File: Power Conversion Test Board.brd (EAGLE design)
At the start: 136.7 x 125.3 mm, 51 parts, among them U1 LM2678, U2 LM2678

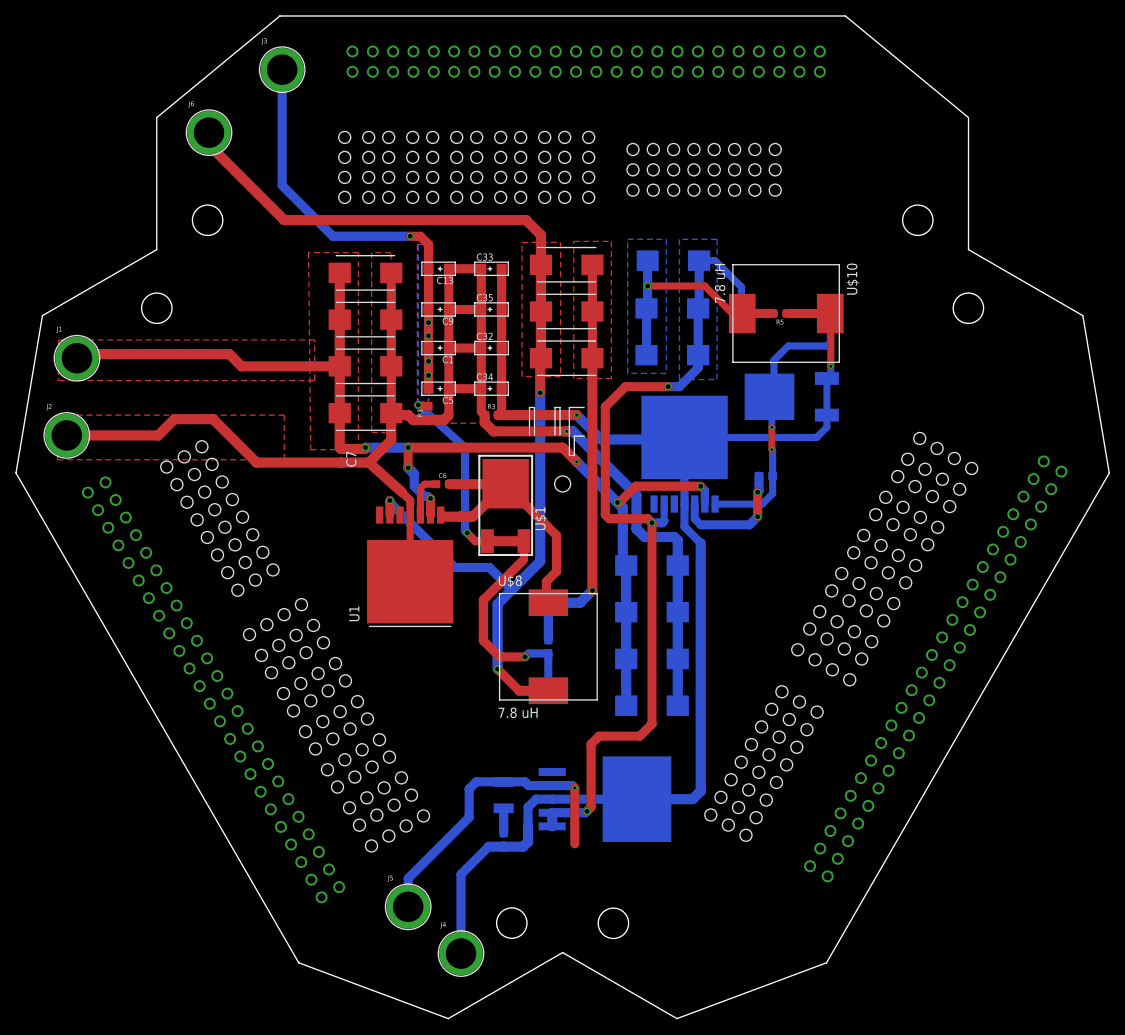
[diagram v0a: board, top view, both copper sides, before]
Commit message: Made some minor changes to the board, just uploading for saving purposes
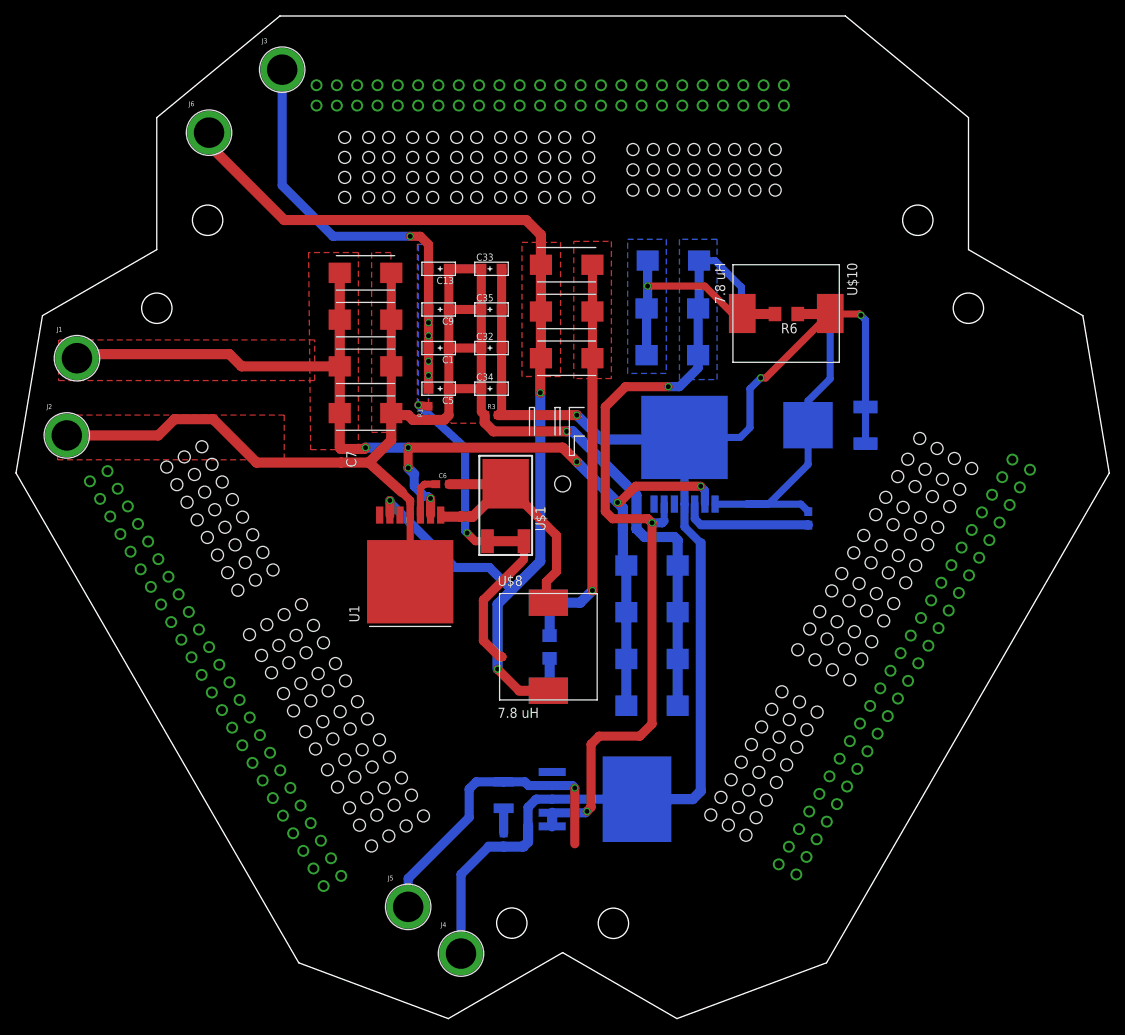
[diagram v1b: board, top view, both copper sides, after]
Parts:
- removed R2, R5: 0, SparkFun-Resistors:0603
- removed U$12, U$13, U$14: PDB_PCB_CONNEC, PDB_PCB_connectors:PDB_PCB
- added R6, R7: 0, audio amplifier example:R1206
- added U$2: PDB_PCB_CONNEC, PDB_PCB_connectors:PDB_PCB_2
- moved C20 7.49 mm to (99.0, 62.5), turned to 90 degrees
- moved U$3 5.99 mm to (102.1, 74.2)
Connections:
- net +12V: now also U$2.+12V1, U$2.+12V10, U$2.+12V11, U$2.+12V12, U$2.+12V13, U$2.+12V14, U$2.+12V15, U$2.+12V16, U$2.+12V17, U$2.+12V18, U$2.+12V19, U$2.+12V2, U$2.+12V20, U$2.+12V21, U$2.+12V22, U$2.+12V23, U$2.+12V24, U$2.+12V25, U$2.+12V26, U$2.+12V27, U$2.+12V28, U$2.+12V29, U$2.+12V3, U$2.+12V30, U$2.+12V31, U$2.+12V32, U$2.+12V33, U$2.+12V34, U$2.+12V35, U$2.+12V36, U$2.+12V37, U$2.+12V38, U$2.+12V39, U$2.+12V4, U$2.+12V40, U$2.+12V41, U$2.+12V42, U$2.+12V43, U$2.+12V44, U$2.+12V45, U$2.+12V46, U$2.+12V47, U$2.+12V48, U$2.+12V49, U$2.+12V5, U$2.+12V50, U$2.+12V51, U$2.+12V52, U$2.+12V53, U$2.+12V54, U$2.+12V55, U$2.+12V56, U$2.+12V57, U$2.+12V58, U$2.+12V59, U$2.+12V6, U$2.+12V60, U$2.+12V61, U$2.+12V62, U$2.+12V63, U$2.+12V64, U$2.+12V65, U$2.+12V66, U$2.+12V67, U$2.+12V68, U$2.+12V69, U$2.+12V7, U$2.+12V70, U$2.+12V71, U$2.+12V72, U$2.+12V8, U$2.+12V9; no longer U$12.+12V1, U$12.+12V10, U$12.+12V11, U$12.+12V12, U$12.+12V13, U$12.+12V14, U$12.+12V15, U$12.+12V16, U$12.+12V17, U$12.+12V18, U$12.+12V19, U$12.+12V2, U$12.+12V20, U$12.+12V21, U$12.+12V22, U$12.+12V23, U$12.+12V24, U$12.+12V3, U$12.+12V4, U$12.+12V5, U$12.+12V6, U$12.+12V7, U$12.+12V8, U$12.+12V9, U$13.+12V1, U$13.+12V10, U$13.+12V11, U$13.+12V12, U$13.+12V13, U$13.+12V14, U$13.+12V15, U$13.+12V16, U$13.+12V17, U$13.+12V18, U$13.+12V19, U$13.+12V2, U$13.+12V20, U$13.+12V21, U$13.+12V22, U$13.+12V23, U$13.+12V24, U$13.+12V3, U$13.+12V4, U$13.+12V5, U$13.+12V6, U$13.+12V7, U$13.+12V8, U$13.+12V9, U$14.+12V1, U$14.+12V10, U$14.+12V11, U$14.+12V12, U$14.+12V13, U$14.+12V14, U$14.+12V15, U$14.+12V16, U$14.+12V17, U$14.+12V18, U$14.+12V19, U$14.+12V2, U$14.+12V20, U$14.+12V21, U$14.+12V22, U$14.+12V23, U$14.+12V24, U$14.+12V3, U$14.+12V4, U$14.+12V5, U$14.+12V6, U$14.+12V7, U$14.+12V8, U$14.+12V9
- net 3.3VGND: now also R6.1; no longer R5.1
- net 5VGND: now also R7.1; no longer R2.1
- net GND: now also U$2.GND1, U$2.GND10, U$2.GND11, U$2.GND12, U$2.GND13, U$2.GND14, U$2.GND15, U$2.GND16, U$2.GND17, U$2.GND18, U$2.GND19, U$2.GND2, U$2.GND20, U$2.GND21, U$2.GND22, U$2.GND23, U$2.GND24, U$2.GND25, U$2.GND26, U$2.GND27, U$2.GND28, U$2.GND29, U$2.GND3, U$2.GND30, U$2.GND31, U$2.GND32, U$2.GND33, U$2.GND34, U$2.GND35, U$2.GND36, U$2.GND37, U$2.GND38, U$2.GND39, U$2.GND4, U$2.GND40, U$2.GND41, U$2.GND42, U$2.GND43, U$2.GND44, U$2.GND45, U$2.GND46, U$2.GND47, U$2.GND48, U$2.GND49, U$2.GND5, U$2.GND50, U$2.GND51, U$2.GND52, U$2.GND53, U$2.GND54, U$2.GND55, U$2.GND56, U$2.GND57, U$2.GND58, U$2.GND59, U$2.GND6, U$2.GND60, U$2.GND61, U$2.GND62, U$2.GND63, U$2.GND64, U$2.GND65, U$2.GND66, U$2.GND67, U$2.GND68, U$2.GND69, U$2.GND7, U$2.GND70, U$2.GND71, U$2.GND72, U$2.GND8, U$2.GND9; no longer U$12.GND10, U$12.GND11, U$12.GND12, U$12.GND13, U$12.GND14, U$12.GND15, U$12.GND16, U$12.GND17, U$12.GND18, U$12.GND19, U$12.GND2, U$12.GND20, U$12.GND21, U$12.GND22, U$12.GND23, U$12.GND24, U$12.GND3, U$12.GND4, U$12.GND5, U$12.GND6, U$12.GND7, U$12.GND8, U$12.GND9, U$13.GND10, U$13.GND11, U$13.GND12, U$13.GND13, U$13.GND14, U$13.GND15, U$13.GND16, U$13.GND17, U$13.GND18, U$13.GND19, U$13.GND2, U$13.GND20, U$13.GND21, U$13.GND22, U$13.GND23, U$13.GND24, U$13.GND3, U$13.GND4, U$13.GND5, U$13.GND6, U$13.GND7, U$13.GND8, U$13.GND9, U$14.GND10, U$14.GND11, U$14.GND12, U$14.GND13, U$14.GND14, U$14.GND15, U$14.GND16, U$14.GND17, U$14.GND18, U$14.GND19, U$14.GND2, U$14.GND20, U$14.GND21, U$14.GND22, U$14.GND23, U$14.GND24, U$14.GND3, U$14.GND4, U$14.GND5, U$14.GND6, U$14.GND7, U$14.GND8, U$14.GND9
- net N$4: now also R6.2; no longer R5.2
- net N$8: now also R7.2; no longer R2.2
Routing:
- net 3.3VGND: track 172.9 -> 186.6 mm, vias 2 -> 3
- net N$7: track 36.6 -> 44.0 mm, vias 2 -> 0
- net 5VGND: track 109.7 -> 103.2 mm, vias 8 -> 7
- net N$2: track 15.6 -> 16.4 mm, vias 2 -> 0
